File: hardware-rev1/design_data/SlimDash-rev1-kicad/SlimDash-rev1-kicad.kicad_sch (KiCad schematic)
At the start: 100 parts, among them U1 TLV73333PDBV, U2 RP2040, U3 W25Q128JVS, Y1 Crystal_GND24

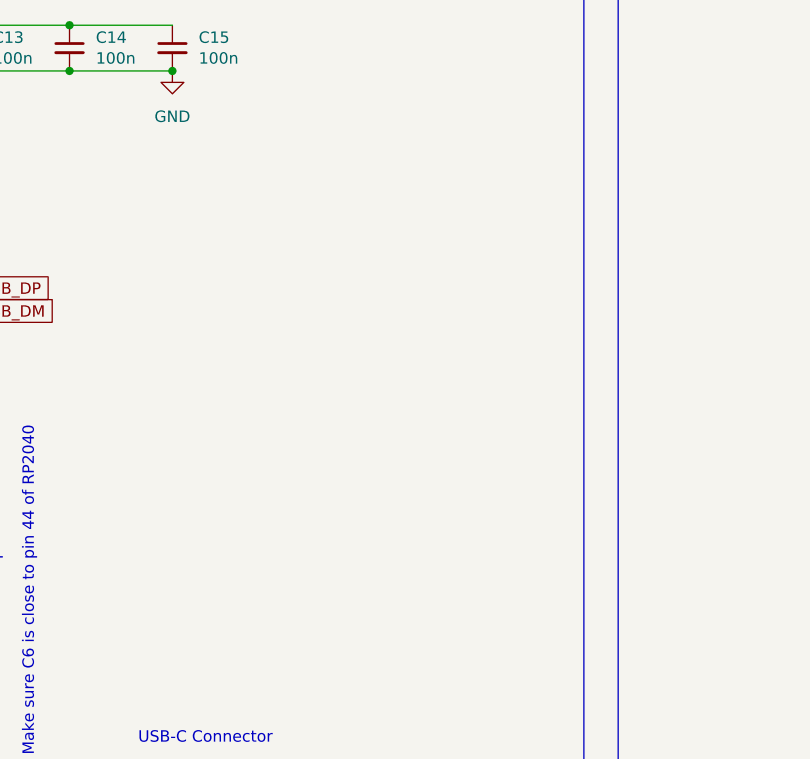
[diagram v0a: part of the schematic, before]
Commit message: add more components to design data
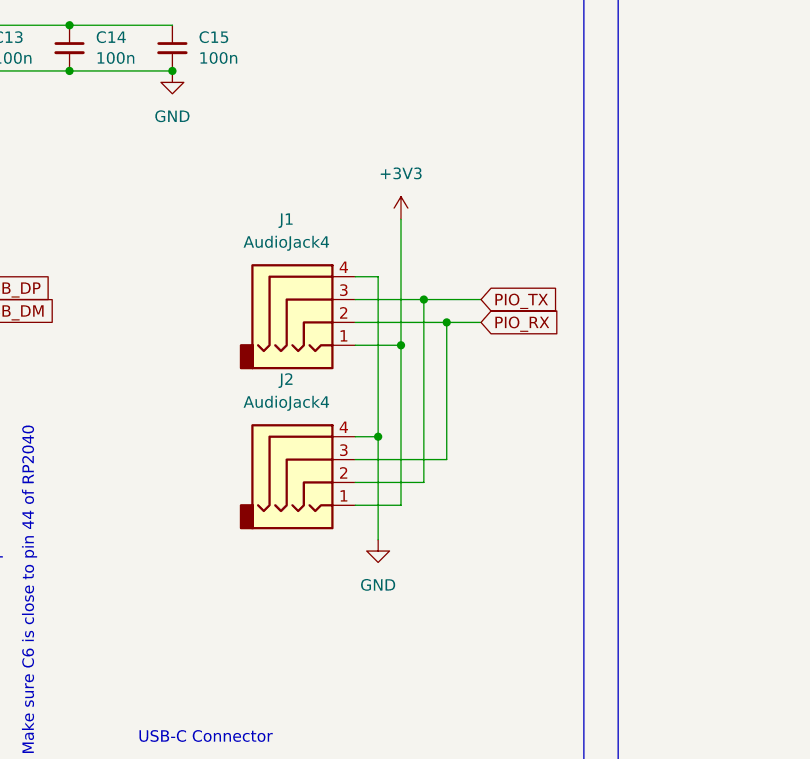
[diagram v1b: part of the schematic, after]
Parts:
- added J1, J2: AudioJack4, Keebio-Parts:TRRS-PJ-320A, symbol Connector_Audio:AudioJack4
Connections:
- net +3V3: now also J1.1, J2.1
- net GND: now also J1.4, J2.4
- new net PIO_RX: J1.2, J2.3
- new net PIO_TX: J1.3, J2.2
